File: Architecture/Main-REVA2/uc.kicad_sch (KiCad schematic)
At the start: 3 parts

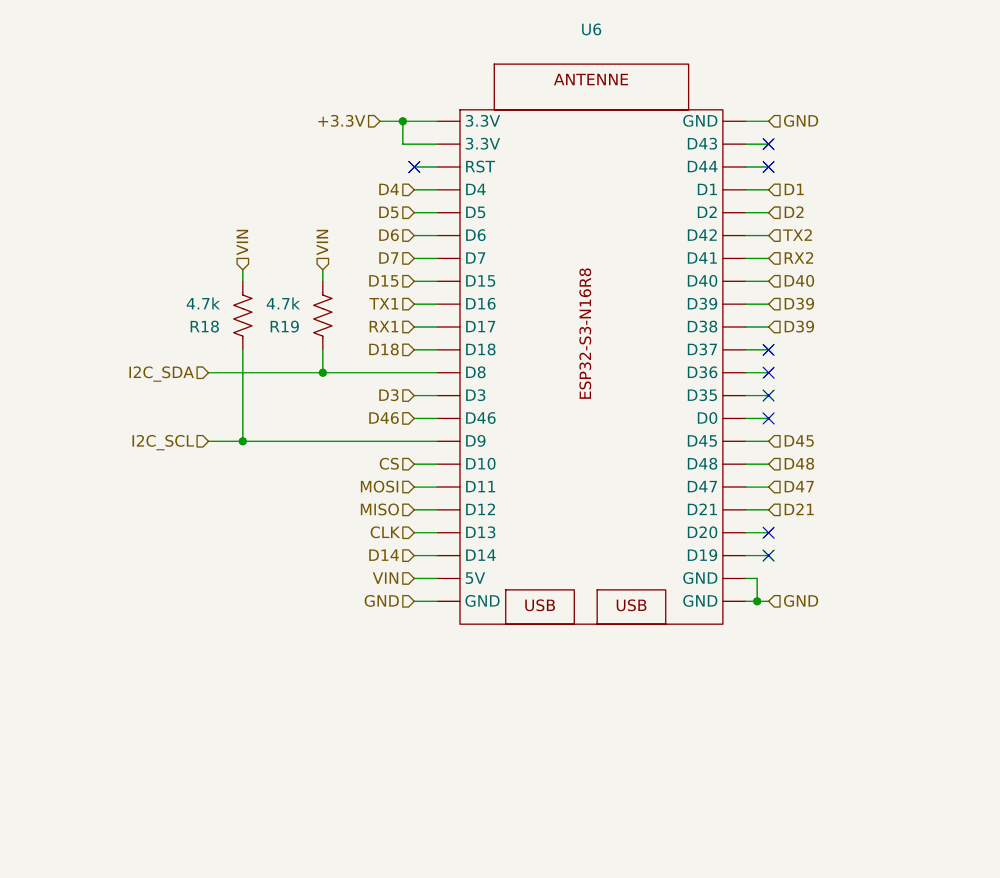
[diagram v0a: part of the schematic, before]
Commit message: Update
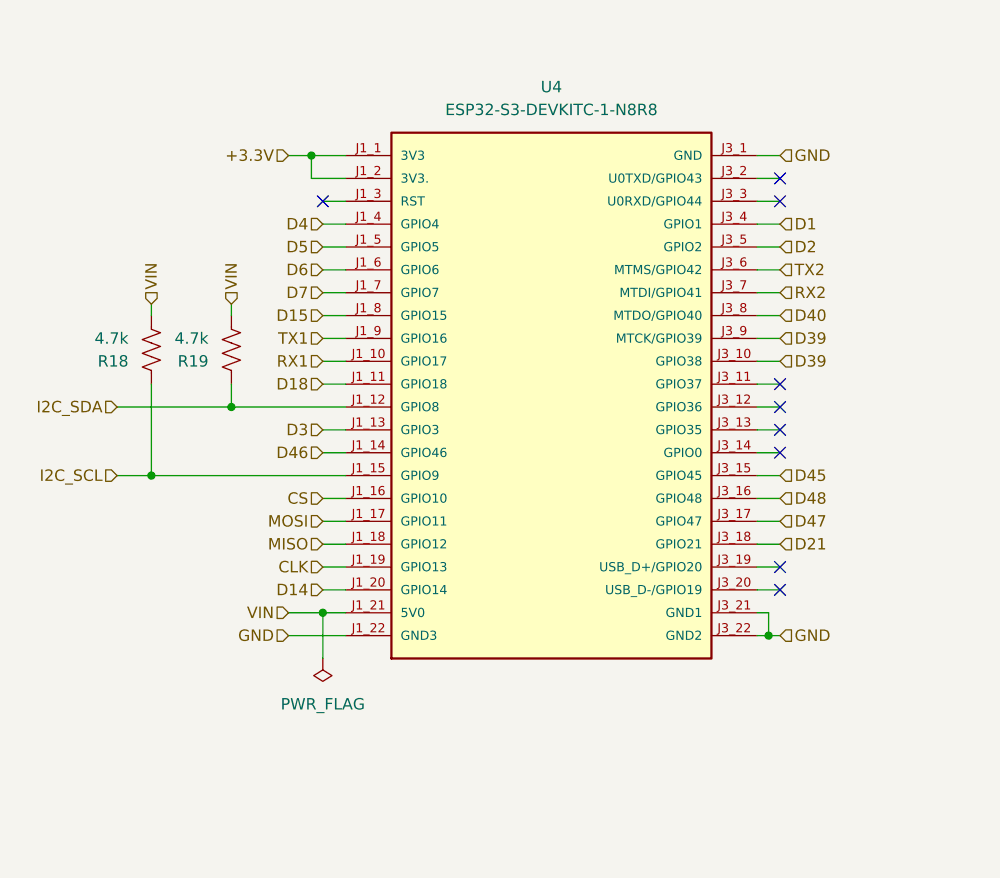
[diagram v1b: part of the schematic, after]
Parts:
- removed U6: ~, symbol MCU:ESP32-S3-N16R8
- added U4: ESP32-S3-DEVKITC-1-N8R8, CollecteurDonne:ESP32-S3-DEVKITC-1-N8R8, symbol ESP32-S3-DEVKITC-1-N8R8:ESP32-S3-DEVKITC-1-N8R8
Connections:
- net +3.3V: now also U4.J1_1 (3V3), U4.J1_2 (3V3.)
- net CLK: now also U4.J1_19 (GPIO13)
- net CS: now also U4.J1_16 (GPIO10)
- net D1: now also U4.J3_4 (GPIO1)
- net D14: now also U4.J1_20 (GPIO14)
- net D15: now also U4.J1_8 (GPIO15)
- net D18: now also U4.J1_11 (GPIO18)
- net D2: now also U4.J3_5 (GPIO2)
- net D21: now also U4.J3_18 (GPIO21)
- net D3: now also U4.J1_13 (GPIO3)
- net D39: now also U4.J3_10 (GPIO38), U4.J3_9 (MTCK/GPIO39)
- net D4: now also U4.J1_4 (GPIO4)
- net D40: now also U4.J3_8 (MTDO/GPIO40)
- net D45: now also U4.J3_15 (GPIO45)
- net D46: now also U4.J1_14 (GPIO46)
- net D47: now also U4.J3_17 (GPIO47)
- net D48: now also U4.J3_16 (GPIO48)
- net D5: now also U4.J1_5 (GPIO5)
- net D6: now also U4.J1_6 (GPIO6)
- net D7: now also U4.J1_7 (GPIO7)
- net GND: now also U4.J1_22 (GND3), U4.J3_1 (GND), U4.J3_21 (GND1), U4.J3_22 (GND2)
- net I2C_SCL: now also U4.J1_15 (GPIO9)
- net I2C_SDA: now also U4.J1_12 (GPIO8)
- net MISO: now also U4.J1_18 (GPIO12)
- net MOSI: now also U4.J1_17 (GPIO11)
- net RX1: now also U4.J1_10 (GPIO17)
- net RX2: now also U4.J3_7 (MTDI/GPIO41)
- net TX1: now also U4.J1_9 (GPIO16)
- net TX2: now also U4.J3_6 (MTMS/GPIO42)
- net VIN: now also U4.J1_21 (5V0)
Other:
- moved on the sheet: R18, R19

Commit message: Update_Sche
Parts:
- R18, R19: footprint (none) -> CollecteurDonne:Résistance L10mm
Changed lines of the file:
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@@
 			)
 		)
-		(property "Footprint" ""
+		(property "Footprint" "CollecteurDonne:Résistance L10mm"
 			(at 72.644 54.356 90)
 			(effects
@@
 			)
 		)
-		(property "Footprint" ""
+		(property "Footprint" "CollecteurDonne:Résistance L10mm"
 			(at 63.754 54.356 90)
 			(effects
